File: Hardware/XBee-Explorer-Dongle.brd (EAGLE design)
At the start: 40.6 x 27.9 mm, 37 parts, among them U2 XBEE-1B3, U3 MIC5219 3.3V, U4 FTS31XS-U

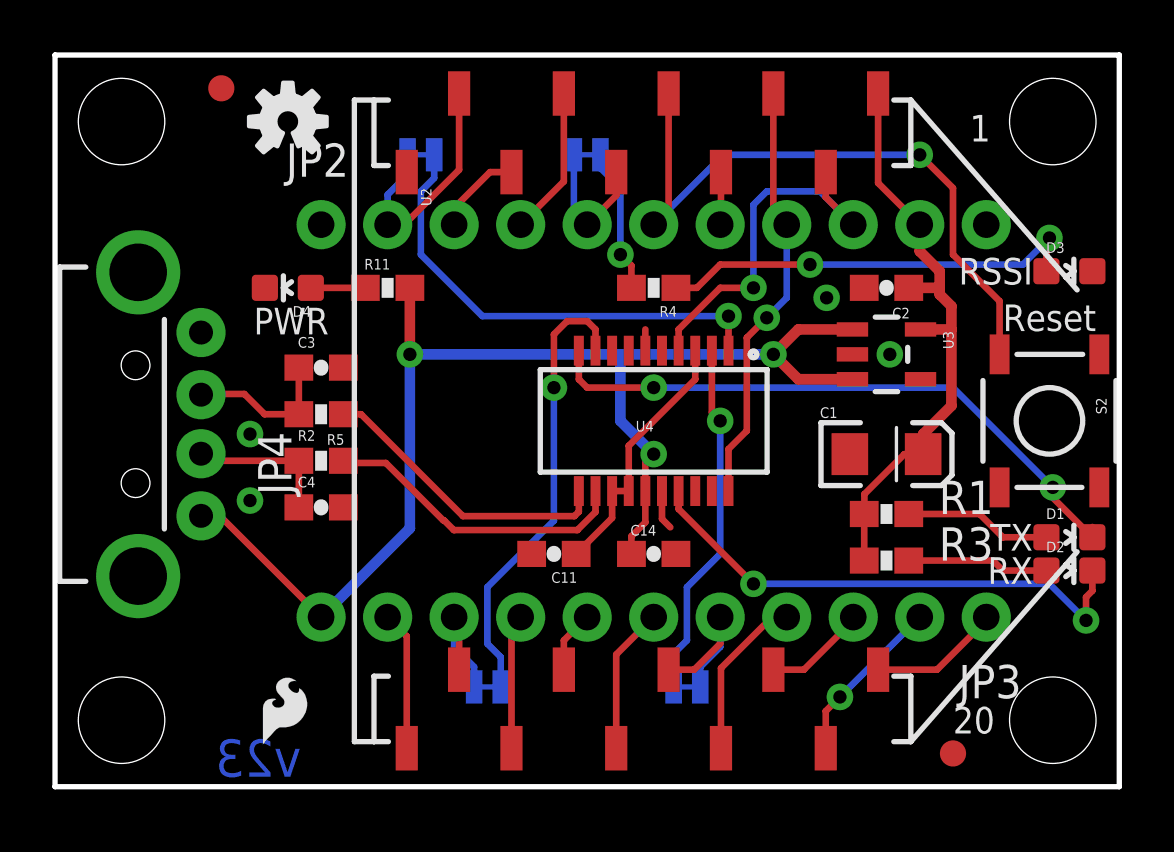
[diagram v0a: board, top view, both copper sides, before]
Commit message: QC checklist items complete.
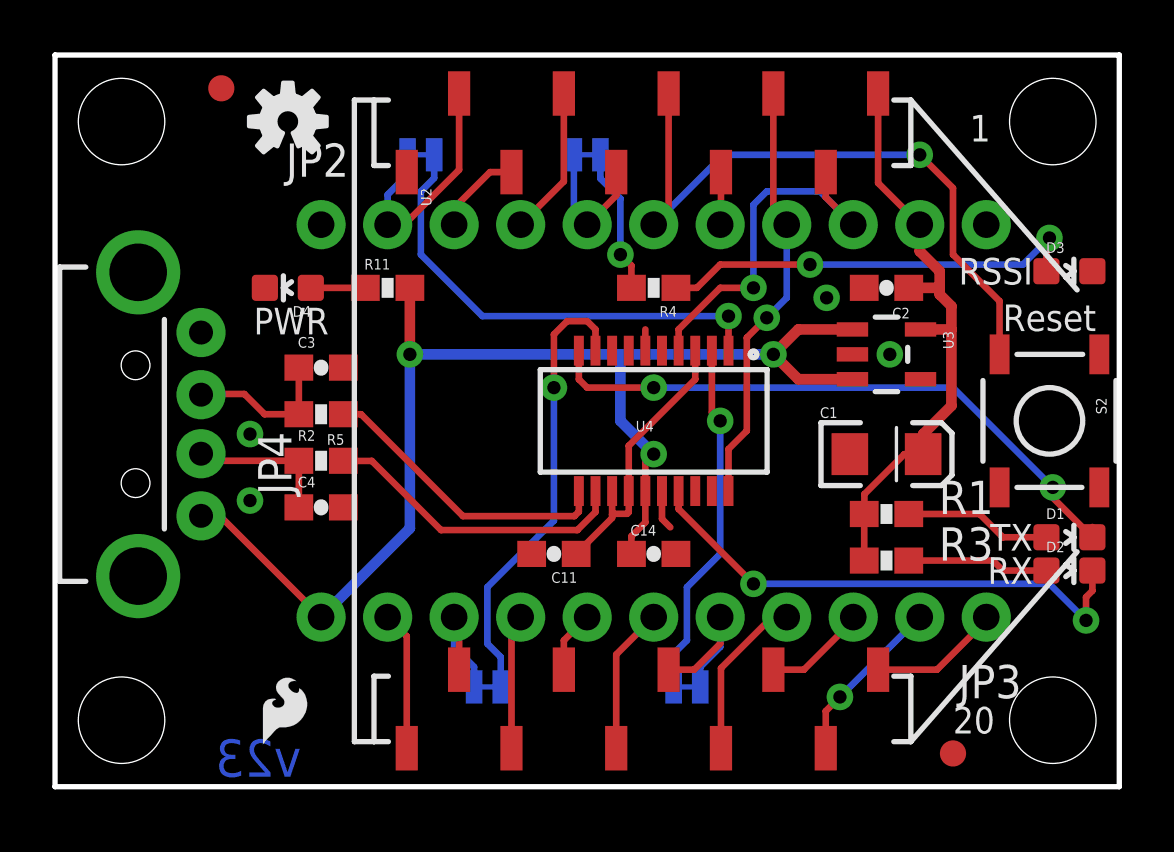
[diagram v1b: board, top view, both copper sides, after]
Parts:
- C11, C14: device SparkFun:0603-CAP -> SparkFun-Capacitors:0603-CAP
- D1: value RED -> GREEN
- D2: value GREEN -> Yellow
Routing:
- net 3V-INT: track 10.0 -> 10.9 mm
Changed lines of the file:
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@@
 </autorouter>
 <elements>
-<element name="C11" library="SparkFun" package="0603-CAP" value="0.1uF" x="19.05" y="8.89" smashed="yes" rot="R180">
+<element name="C11" library="SparkFun-Capacitors" package="0603-CAP" value="0.1uF" x="19.05" y="8.89" smashed="yes" rot="R180">
 <attribute name="NAME" x="19.939" y="8.1915" size="0.4064" layer="25" rot="R180"/>
-<attribute name="VALUE" x="16.1925" y="8.763" size="0.4064" layer="27"/>
+<attribute name="VALUE" value="0.1uF" x="16.1925" y="8.763" size="0.4064" layer="27"/>
+<attribute name="PROD_ID" value="CAP-00810" x="19.05" y="8.89" size="1.778" layer="27" rot="R180" display="off"/>
 </element>
 <element name="R11" library="SparkFun-Resistors" package="0603-RES" value="1K" x="12.7" y="19.05" smashed="yes">
@@
 <attribute name="PROD_ID" value="RES-07856" x="12.7" y="19.05" size="1.778" layer="27" display="off"/>
 </element>
-<element name="C14" library="SparkFun" package="0603-CAP" value="0.1uF" x="22.86" y="8.89" smashed="yes">
+<element name="C14" library="SparkFun-Capacitors" package="0603-CAP" value="0.1uF" x="22.86" y="8.89" smashed="yes">
 <attribute name="NAME" x="21.971" y="9.5885" size="0.4064" layer="25"/>
-<attribute name="VALUE" x="19.8755" y="8.636" size="0.4064" layer="27"/>
+<attribute name="VALUE" value="0.1uF" x="19.8755" y="8.636" size="0.4064" layer="27"/>
+<attribute name="PROD_ID" value="CAP-00810" x="22.86" y="8.89" size="1.778" layer="27" display="off"/>
 </element>
 <element name="R1" library="SparkFun-Resistors" package="0603-RES" value="1K" x="31.75" y="10.414" smashed="yes">
@@
 <element name="SJ3" library="SparkFun-Passives" package="SJ_2S-TRACE" value="RSSI" x="16.51" y="3.81" rot="MR0"/>
 <element name="SJ4" library="SparkFun-Passives" package="SJ_2S-TRACE" value="RSSI" x="13.97" y="24.13" rot="MR0"/>
-<element name="D1" library="SparkFun-LED" package="LED-0603" value="RED" x="38.735" y="9.525" rot="R270">
-<attribute name="PROD_ID" value="DIO-00819" x="38.735" y="9.525" size="1.778" layer="27" font="vector" ratio="15" rot="R270" display="off"/>
-</element>
-<element name="D2" library="SparkFun-LED" package="LED-0603" value="GREEN" x="38.735" y="8.255" rot="R270">
-<attribute name="PROD_ID" value="DIO-00821" x="38.735" y="8.255" size="1.778" layer="27" font="vector" ratio="15" rot="R270" display="off"/>
+<element name="D1" library="SparkFun-LED" package="LED-0603" value="GREEN" x="38.735" y="9.525" rot="R270">
+<attribute name="PROD_ID" value="DIO-00821" x="38.735" y="9.525" size="1.778" layer="27" font="vector" ratio="15" rot="R270" display="off"/>
+</element>
+<element name="D2" library="SparkFun-LED" package="LED-0603" value="Yellow" x="38.735" y="8.255" rot="R270">
+<attribute name="PROD_ID" value="DIO-09003" x="38.735" y="8.255" size="1.778" layer="27" font="vector" ratio="15" rot="R270" display="off"/>
 </element>
 <element name="D3" library="SparkFun-LED" package="LED-0603" value="GREEN" x="38.735" y="19.685" rot="R270">
@@
 <contactref element="U4" pad="3"/>
 <contactref element="U4" pad="13"/>
-<wire x1="21.9075" y1="11.2903" x2="21.2725" y2="11.2903" width="0.254" layer="1"/>
 <wire x1="21.9075" y1="11.2903" x2="21.9075" y2="13.0175" width="0.254" layer="1"/>
 <wire x1="24.4475" y1="16.6497" x2="24.4475" y2="15.5575" width="0.254" layer="1"/>
 <wire x1="24.4475" y1="15.5575" x2="21.9075" y2="13.0175" width="0.254" layer="1"/>
-<wire x1="21.2725" y1="11.2903" x2="21.2725" y2="10.2625" width="0.254" layer="1"/>
+<wire x1="21.2725" y1="11.2903" x2="21.2725" y2="10.398759375" width="0.254" layer="1"/>
+<wire x1="21.2725" y1="10.398759375" x2="21.2725" y2="10.2625" width="0.254" layer="1"/>
 <wire x1="21.2725" y1="10.2625" x2="19.9" y2="8.89" width="0.254" layer="1"/>
+<wire x1="21.9075" y1="11.2903" x2="21.9075" y2="10.482578125" width="0.254" layer="1"/>
+<wire x1="21.9075" y1="10.482578125" x2="21.846540625" y2="10.42161875" width="0.254" layer="1"/>
+<wire x1="21.846540625" y1="10.42161875" x2="21.295359375" y2="10.42161875" width="0.254" layer="1"/>
+<wire x1="21.295359375" y1="10.42161875" x2="21.2725" y2="10.398759375" width="0.254" layer="1"/>
 </signal>
 <signal name="N$3">
@@
 <wire x1="20.6375" y1="11.2903" x2="20.6375" y2="10.4902" width="0.254" layer="1"/>
 <wire x1="20.6375" y1="10.4902" x2="19.94661875" y2="9.79931875" width="0.254" layer="1"/>
-<wire x1="19.94661875" y1="9.79931875" x2="15.2273" y2="9.79931875" width="0.254" layer="1"/>
-<wire x1="15.2273" y1="9.79931875" x2="14.856459375" y2="10.170159375" width="0.254" layer="1"/>
-<wire x1="14.856459375" y1="10.170159375" x2="14.82598125" y2="10.170159375" width="0.254" layer="1"/>
-<wire x1="14.82598125" y1="10.170159375" x2="12.633959375" y2="12.36218125" width="0.254" layer="1"/>
-<wire x1="12.633959375" y1="12.36218125" x2="11.09381875" y2="12.36218125" width="0.254" layer="1"/>
+<wire x1="19.94661875" y1="9.79931875" x2="14.73961875" y2="9.79931875" width="0.254" layer="1"/>
 <wire x1="11.09381875" y1="12.36218125" x2="11.01" y2="12.446" width="0.254" layer="1"/>
+<wire x1="14.73961875" y1="9.79931875" x2="12.09801875" y2="12.44091875" width="0.254" layer="1"/>
+<wire x1="12.09801875" y1="12.44091875" x2="11.01508125" y2="12.44091875" width="0.254" layer="1"/>
+<wire x1="11.01508125" y1="12.44091875" x2="11.01" y2="12.446" width="0.254" layer="1"/>
 </signal>
 <signal name="N$6">
@@
 <contactref element="R4" pad="2"/>
 <contactref element="SJ1" pad="2"/>
-<wire x1="20.828" y1="24.13" x2="20.828" y2="23.622" width="0.254" layer="16"/>
-<wire x1="20.828" y1="23.622" x2="21.59" y2="22.86" width="0.254" layer="16"/>
-<wire x1="21.59" y1="22.86" x2="21.59" y2="20.32" width="0.254" layer="16"/>
 <via x="21.59" y="20.32" extent="1-16" drill="0.508"/>
 <wire x1="21.59" y1="20.32" x2="22.01" y2="19.9" width="0.254" layer="1"/>
 <wire x1="22.01" y1="19.05" x2="22.01" y2="19.9" width="0.254" layer="1"/>
+<wire x1="21.59" y1="20.32" x2="21.59" y2="22.458678125" width="0.254" layer="16"/>
+<wire x1="21.59" y1="22.458678125" x2="20.825459375" y2="23.22321875" width="0.254" layer="16"/>
+<wire x1="20.825459375" y1="23.22321875" x2="20.825459375" y2="24.127459375" width="0.254" layer="16"/>
+<wire x1="20.825459375" y1="24.127459375" x2="20.828" y2="24.13" width="0.254" layer="16"/>
 </signal>
 <signal name="RTS_XBEE">
